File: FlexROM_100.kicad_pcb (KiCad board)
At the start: 2 copper layers, 17.8 x 35.6 mm, 6 parts, among them J1 LH535618 DIP LEGS, U1 28C256

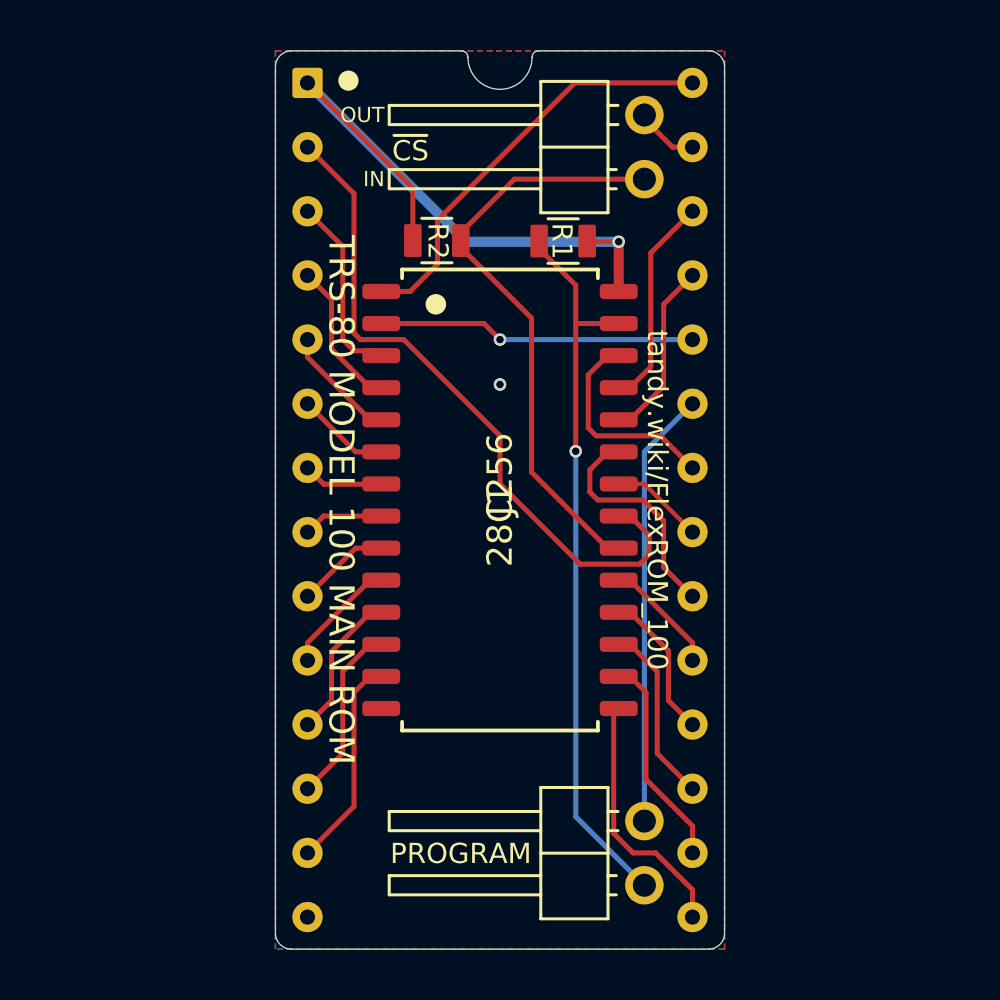
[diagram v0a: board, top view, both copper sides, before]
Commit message: various minor cleanups
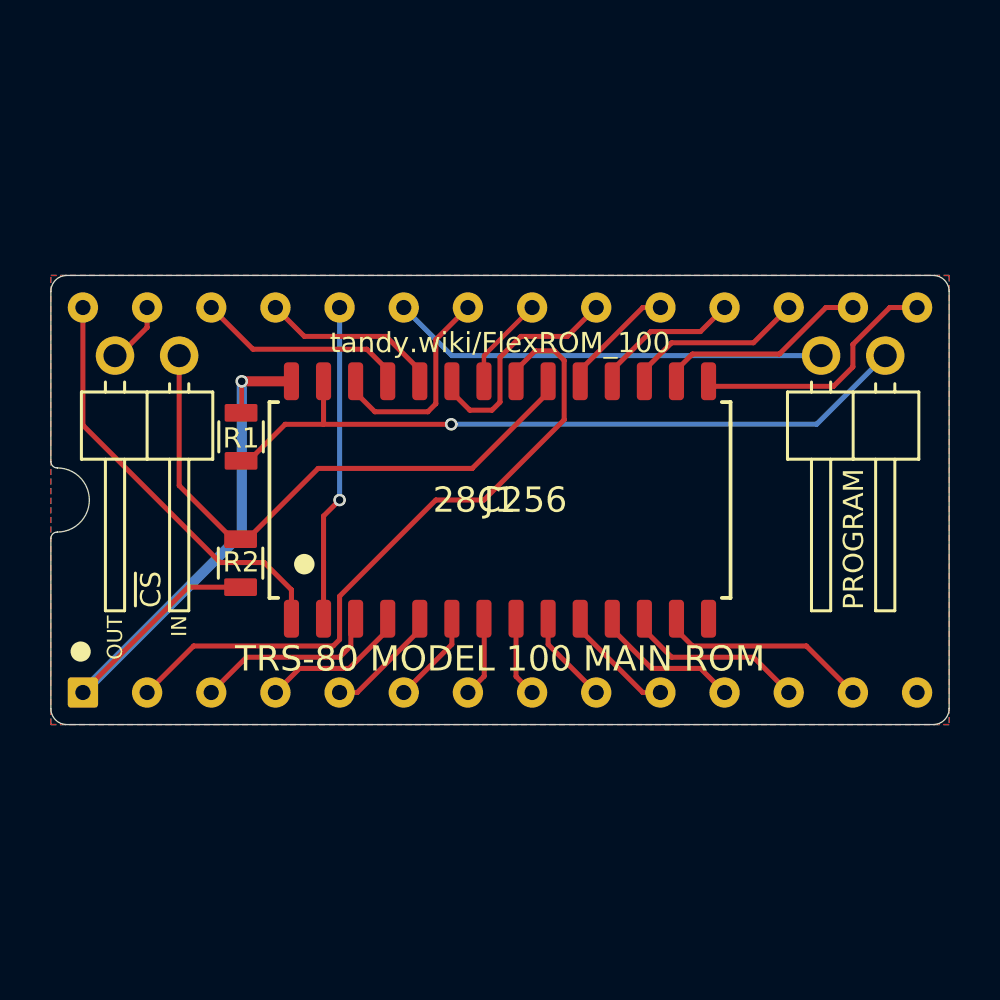
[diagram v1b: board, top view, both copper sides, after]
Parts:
- moved JP2 23.0 mm to (165.2, 94.3), turned to -90 degrees
- moved JP1 19.7 mm to (137.3, 94.3), turned to -90 degrees
- moved R2 14.9 mm to (139.7, 102.5), turned to -90 degrees
- moved R1 14.9 mm to (139.8, 97.5), turned to -90 degrees
- turned J1 to 90 degrees
- turned U1 to 90 degrees
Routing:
- net GND: vias 1 -> 0
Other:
- board size 17.8 x 35.6 mm -> 35.6 x 17.8 mm
- board text added: "${TITLE} ${REVISION} ${COMMENT2}"
- board text added: "R1: ${00000000-0000-0000-0000-00005fbb7cd5:VALUE} Legs: TE 1544210"
- board text added: "REX_Classic main ROM support: ~{CS}_OUT to REX TP1 to boot REX main rom ~{CS}_OUT to ~{CS}_IN to boot internal main rom"
- board text removed: "Connect ~{CS} OUT to REX TP1. Leave ~{CS} IN unconnected."
- board text removed: "If REX is later removed, connect ~{CS} OUT to ~{CS} IN."
- board text removed: "Install a shunt on ~{CS}, or, install wires as above,"
- board text removed: "Legs: TE 1544210"
- board text removed: "R1, R2: 47k"
- board text removed: "REX can then be added later without disassembling."
- board text removed: "Run 2 wires from ~{CS} IN & ~{CS} OUT to Option ROM compartment."
- board text removed: "To use REX Main ROM feature:"
- board text removed: "To use without REX:"
- board text removed: "and connect them to each other in the Option ROM compartment."
